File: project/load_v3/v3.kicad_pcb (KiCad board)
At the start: 2 copper layers, 148.9 x 22.9 mm, 133 parts, among them IC1 ATMEGA328-P, P1 12VAC, P10 overheat, P11 G, P12 opto, P13 tac_auto, P14 pwr, P15 overheat, P16 g, P2 NGUON, P3 SAC, P4 DS, P5 CONN_01X02, P6 button, P7 UART, P8 FAN, P9 7-seg, Q1 Q_NPN_BCE, Q2 Q_NPN_BCE, Q3 Q_NPN_BCE, Q4 2n222, Q5 2n222, Q6 Q_NMOS_GDS, Q7 Q_NMOS_GDS, SW1 reset, U1 LM7812CT, U10 PC817, U2 LM7805CT, U3 ICL7660, U4 TL431, U5 LM324N, U6 LM358, U7 LM7812CT, U8 LM358, U9 PC817, Y1 16MHz

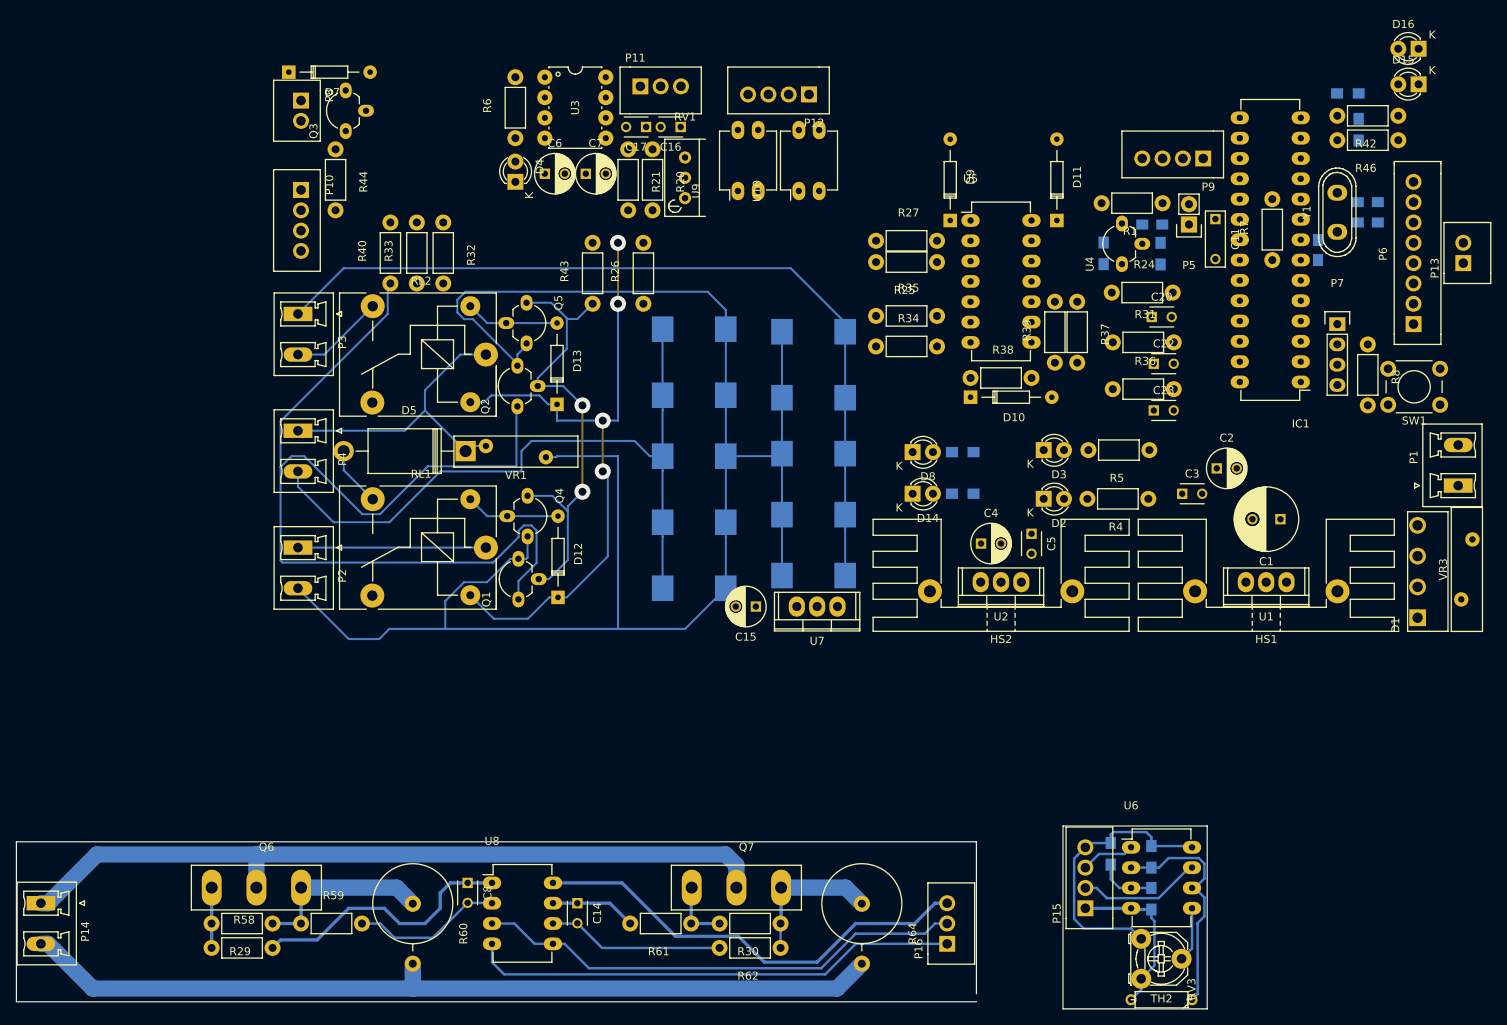
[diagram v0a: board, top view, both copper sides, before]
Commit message: a
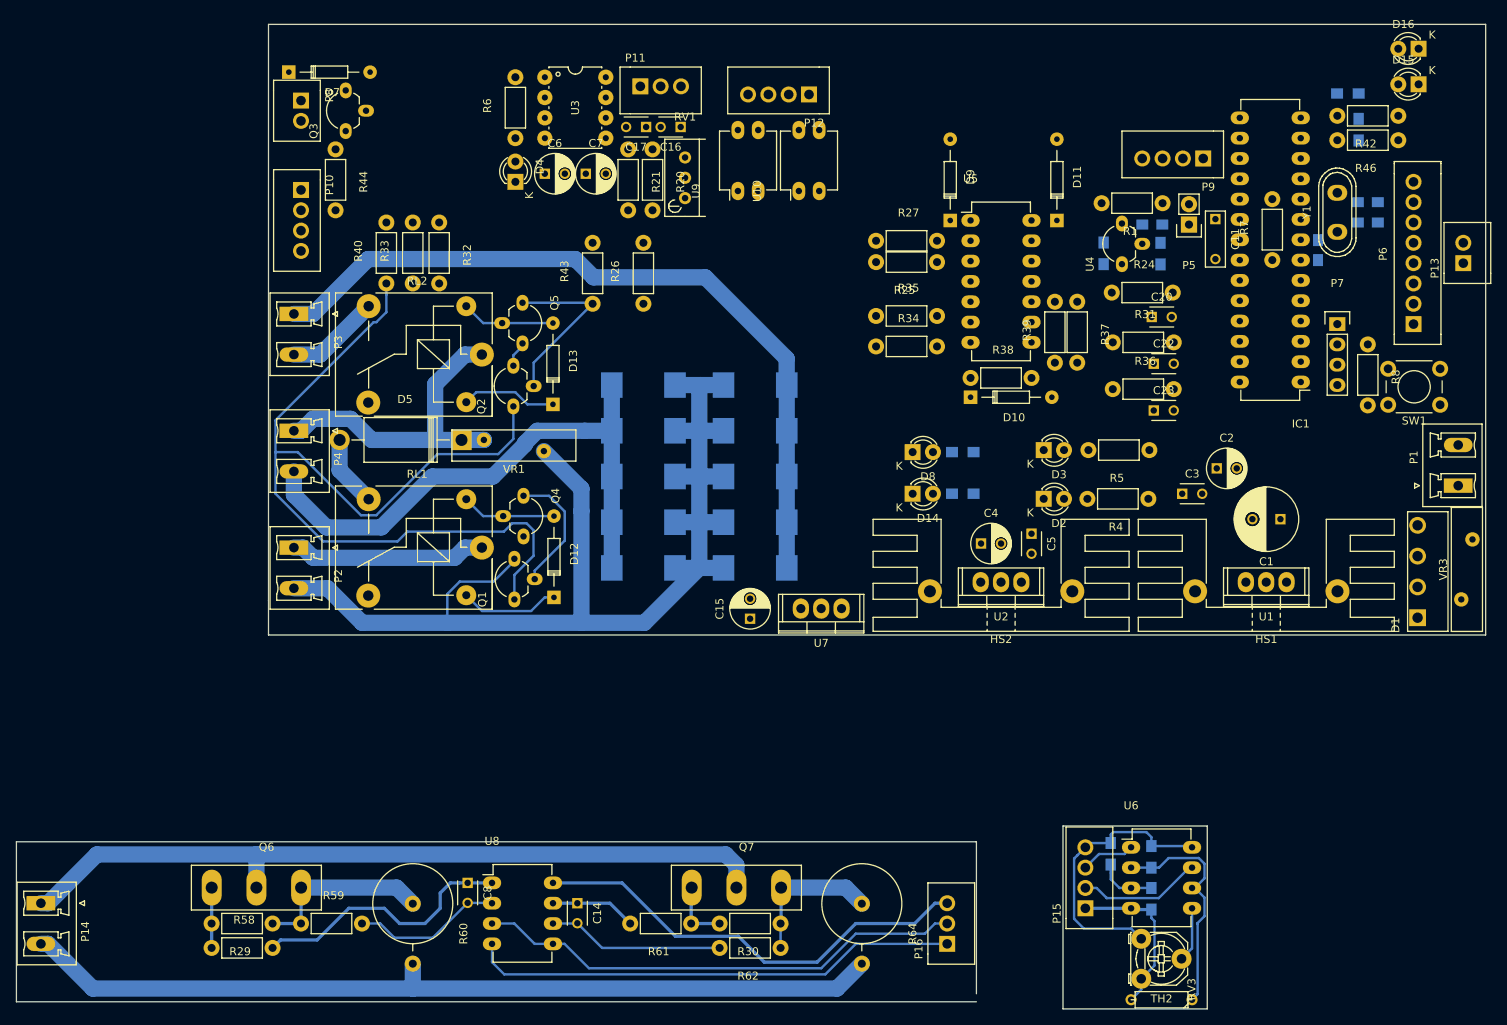
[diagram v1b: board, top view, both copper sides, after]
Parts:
- moved R18 9.89 mm to (106.0, 199.4)
- moved R9 9.44 mm to (92.1, 199.4)
- moved R17 8.39 mm to (106.0, 205.1)
- moved R16 7.84 mm to (106.0, 210.8)
- moved R10 7.75 mm to (92.1, 205.1)
- moved R14 7.36 mm to (106.0, 222.2)
- moved R15 7.36 mm to (106.0, 216.5)
- moved R11 6.84 mm to (92.1, 210.8)
- moved R13 6.84 mm to (92.1, 222.2)
- moved R12 6.35 mm to (92.1, 216.5)
- moved C15 1.69 mm to (105.4, 228.6), turned to 90 degrees
- moved D5 1.49 mm to (69.3, 206.2)
- moved VR1 0.80 mm to (72.1, 206.2)
- moved U7 0.57 mm to (114.3, 227.3)
- moved P2 0.51 mm to (48.4, 219.7)
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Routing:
- net N-: track 252.8 -> 171.8 mm
- net 12Vrelay: track 117.6 -> 59.7 mm, vias 4 -> 0
- net onN: track 57.0 -> 38.1 mm, vias 2 -> 0
- net S: track 197.5 -> 181.6 mm
- net S-: track 106.6 -> 95.8 mm
- net Net-(Q1-Pad1): track 127.7 -> 119.8 mm
- net rN+: track 7.52 -> 8.91 mm
- net N+: track 23.5 -> 24.5 mm
- net D: track 135.9 -> 136.8 mm
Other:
- board size 148.9 x 22.9 mm -> 183.7 x 123.1 mm
- net class Default: clearance 0.25 -> 0.35
- rule trace_clearance: 0.25 -> 0.35
